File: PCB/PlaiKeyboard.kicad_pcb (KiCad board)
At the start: 2 copper layers, 370 x 140 mm, 170 parts, among them SW10 SW_Push_45deg, SW11 SW_Push_45deg, SW12 SW_Push_45deg, SW13 SW_Push_45deg, SW14 SW_Push_45deg, SW15 SW_Push_45deg, SW16 SW_Push_45deg, SW17 SW_Push_45deg, SW18 SW_Push_45deg, SW19 SW_Push_45deg, SW2 SW_Push_45deg, SW20 SW_Push_45deg, SW21 SW_Push_45deg, SW22 SW_Push_45deg, SW23 SW_Push_45deg, SW24 SW_Push_45deg, SW25 SW_Push_45deg, SW26 SW_Push_45deg, SW27 SW_Push_45deg, SW28 SW_Push_45deg, SW29 SW_Push_45deg, SW3 SW_Push_45deg, SW30 SW_Push_45deg, SW31 SW_Push_45deg, SW32 SW_Push_45deg, SW33 SW_Push_45deg, SW34 SW_Push_45deg, SW35 SW_Push_45deg, SW36 SW_Push_45deg, SW37 SW_Push_45deg, SW38 SW_Push_45deg, SW39 SW_Push_45deg, SW4 SW_Push_45deg, SW40 SW_Push_45deg, SW41 SW_Push_45deg, SW42 SW_Push_45deg, SW43 SW_Push_45deg, SW44 SW_Push_45deg, SW45 SW_Push_45deg, SW46 SW_Push_45deg, SW47 SW_Push_45deg, SW48 SW_Push_45deg, SW49 SW_Push_45deg, SW5 SW_Push_45deg, SW50 SW_Push_45deg, SW51 SW_Push_45deg, SW52 SW_Push_45deg, SW53 SW_Push_45deg, SW54 SW_Push_45deg, SW55 SW_Push_45deg, SW56 SW_Push_45deg, SW57 SW_Push_45deg, SW58 SW_Push_45deg, SW59 SW_Push_45deg, SW6 SW_Push_45deg, SW60 SW_Push_45deg, SW61 SW_Push_45deg, SW62 SW_Push_45deg, SW63 SW_Push_45deg, SW64 SW_Push_45deg, SW65 SW_Push_45deg, SW66 SW_Push_45deg, SW67 SW_Push_45deg, SW68 SW_Push_45deg, SW69 SW_Push_45deg, SW7 SW_Push_45deg, SW70 SW_Push_45deg, SW71 SW_Push_45deg, SW72 SW_Push_45deg, SW73 SW_Push_45deg, SW74 SW_Push_45deg, SW75 SW_Push_45deg, SW76 SW_Push_45deg, SW77 SW_Push_45deg, SW78 RotaryEncoder_Switch, SW79 SW_Push_45deg, SW8 SW_Push_45deg, SW80 SW_Push_45deg, SW81 SW_Push_45deg, SW82 SW_Push_45deg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

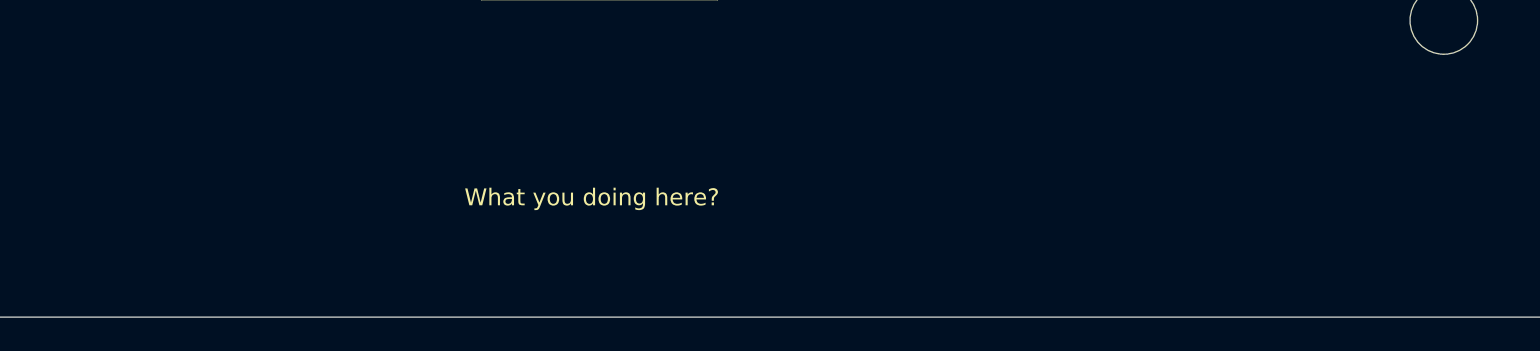
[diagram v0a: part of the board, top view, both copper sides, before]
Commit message: New Changes
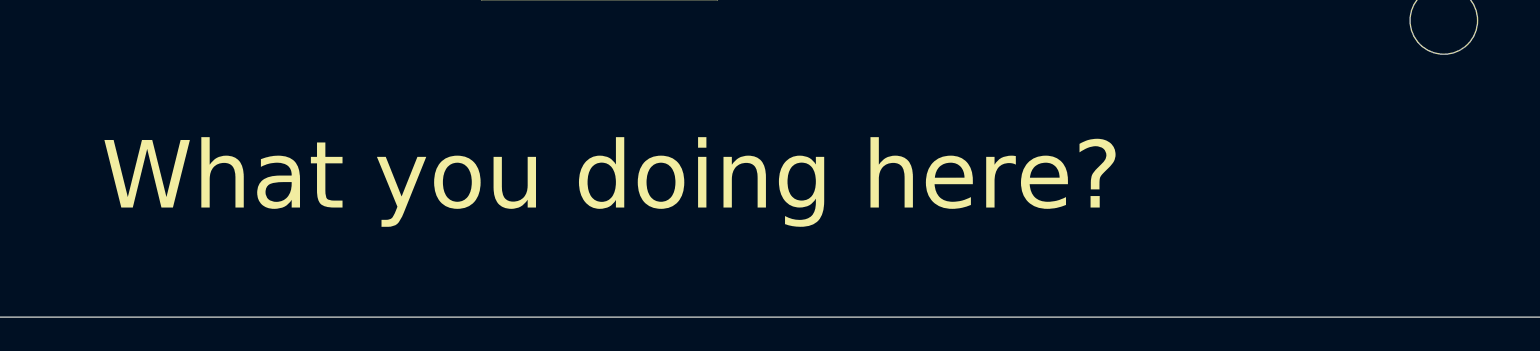
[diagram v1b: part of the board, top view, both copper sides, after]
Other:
- board text added: "Roman S"
